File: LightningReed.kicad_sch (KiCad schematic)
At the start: 71 parts, among them P1 Conn_WallPlug, Q1 NCE65T180D, Q2 2N7002, Q3 Q_NMOS_GDS, Q4 2N7002, Q5 2N7002K, Q6 2N7002K, U1 UCC28056, U2 78L05S, U3 LMC7111, U4 UCC28780

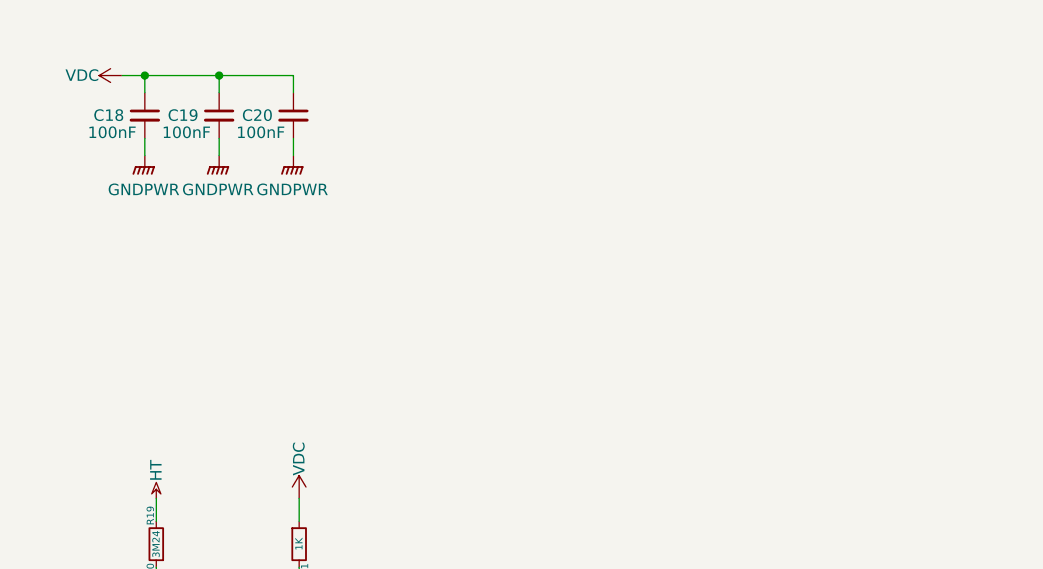
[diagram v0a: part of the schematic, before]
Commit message: Transformer
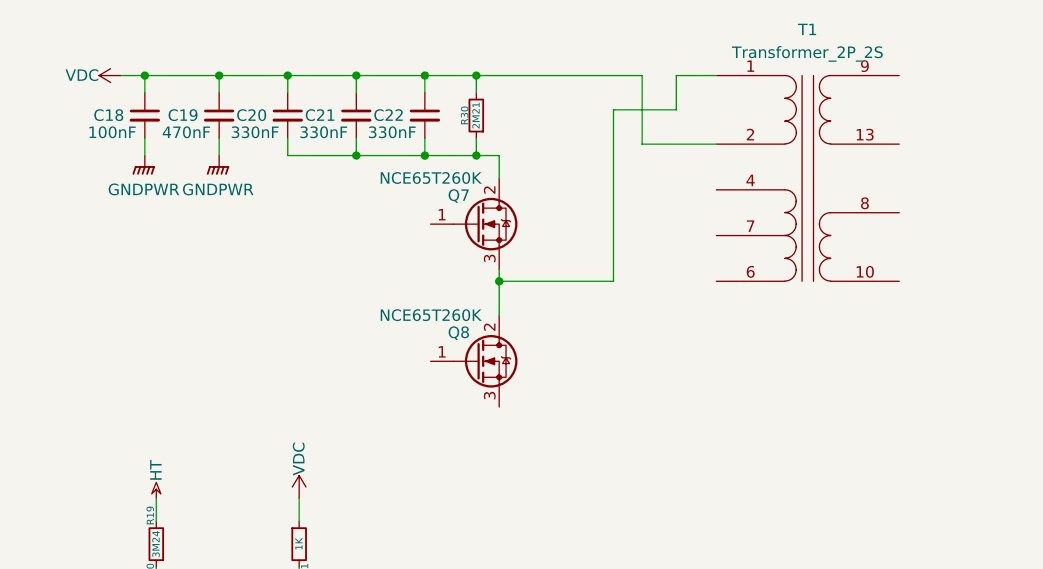
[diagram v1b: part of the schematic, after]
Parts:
- added C21, C22: 330nF, symbol Device:C_Small
- added Q7, Q8: NCE65T260K, symbol Device:Q_NMOS_GDS
- added R30: 2M21, symbol Device:R_Small
- added T1: Transformer_2P_2S, symbol LightningReed:Transformer_2P_2S
- C19: value 100nF -> 470nF
- C20: value 100nF -> 330nF
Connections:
- net GNDPWR: no longer C20.2
- net VDC: now also C21.1, C22.1, R30.2, T1.2 (AB)
- new net: C20.2, C21.2, C22.2, Q7.2 (D), R30.1
- new net: Q7.3 (S), Q8.2 (D), T1.1 (AA)

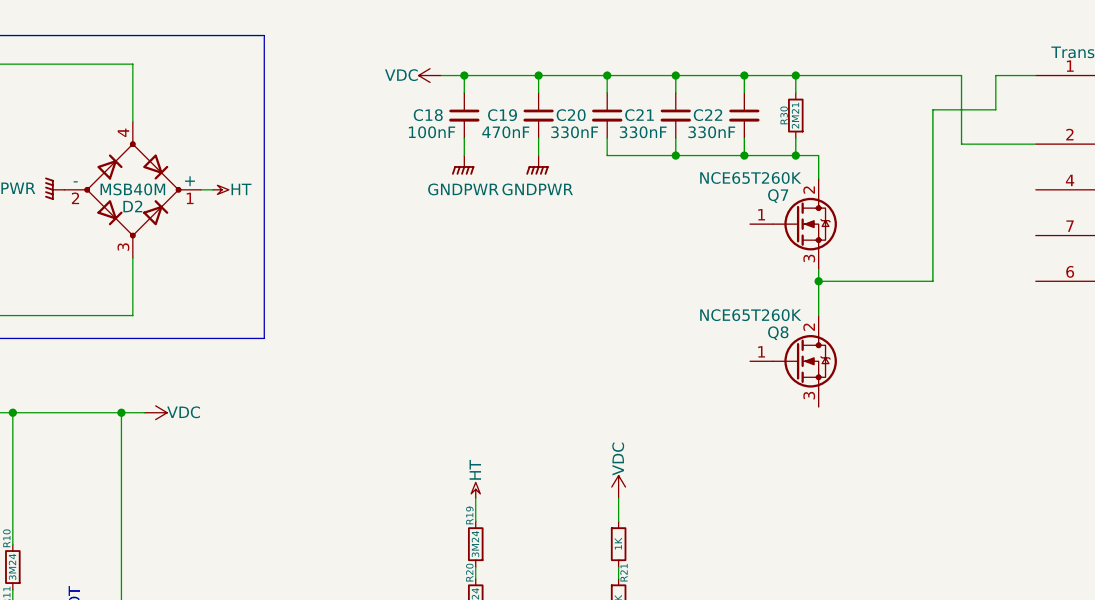
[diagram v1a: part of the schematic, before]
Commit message: HB Driver
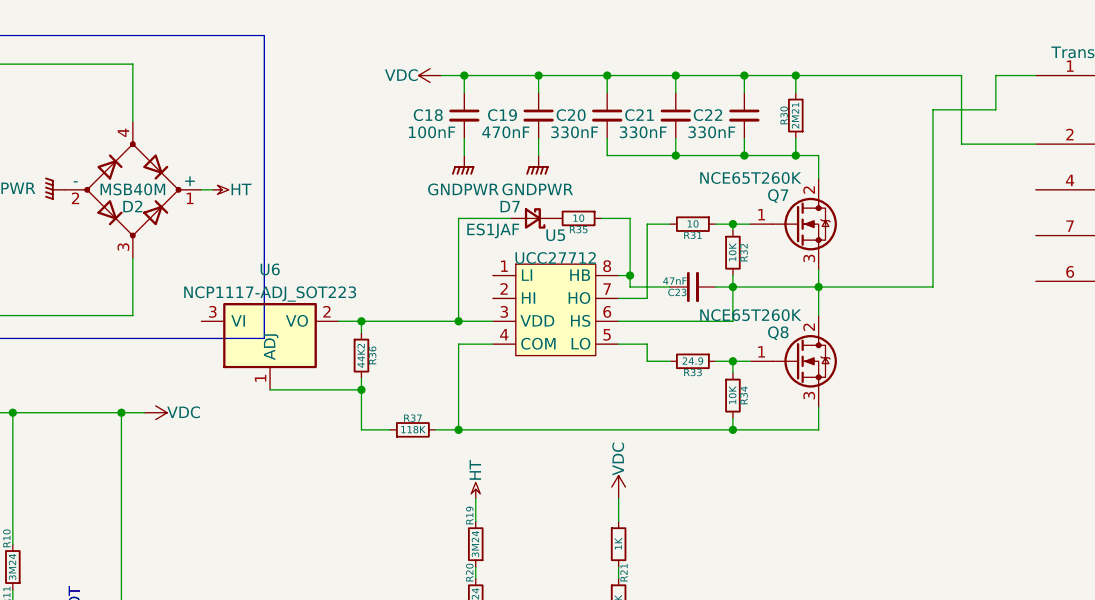
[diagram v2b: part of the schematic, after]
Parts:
- added C23: 47nF, symbol Device:C_Small
- added D7: ES1JAF, symbol Device:D_Schottky_Small
- added R31, R35: 10, symbol Device:R_Small
- added R32, R34: 10K, symbol Device:R_Small
- added R33: 24.9, symbol Device:R_Small
- added R36: 44K2, symbol Device:R_Small
- added R37: 118K, symbol Device:R_Small
- added U5: UCC27712, symbol LightningReed:UCC27712
- added U6: NCP1117-ADJ_SOT223, Package_TO_SOT_SMD:SOT-223-3_TabPin2, symbol Regulator_Linear:NCP1117-ADJ_SOT223
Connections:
- net at Q7.3 (S), Q8.2 (D), T1.1 (AA): now also C23.2, R32.2, U5.6 (HS)
- net at Q8.1 (G): now also R33.1, R34.1
- net at Q8.3 (S): now also R34.2, R37.2, U5.4 (COM)
- net at Q7.1 (G): now also R31.1, R32.1
- new net: C23.1, R35.1, U5.8 (HB)
- new net: R36.2, R37.1, U6.1 (ADJ)
- new net: D7.2 (A), R36.1, U5.3 (VDD), U6.2 (VO)
- new net: R33.2, U5.5 (LO)
- new net: R31.2, U5.7 (HO)
- new net: D7.1 (K), R35.2
